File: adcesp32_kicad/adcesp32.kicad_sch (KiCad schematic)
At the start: 33 parts, among them IC1 PCM1862DBT, J1 AudioJack4, J2 USB_C_Receptacle_USB2.0_16P, J3 RCJ-2112, J4 Conn_01x05_Pin, J5 Conn_01x05_Pin, J6 Conn_01x04_Pin, J7 Conn_01x04_Pin, SW1 SW_Push, SW2 SW_Push, U1 ESP32-S3-WROOM-1, U2 AMS1117-3.3

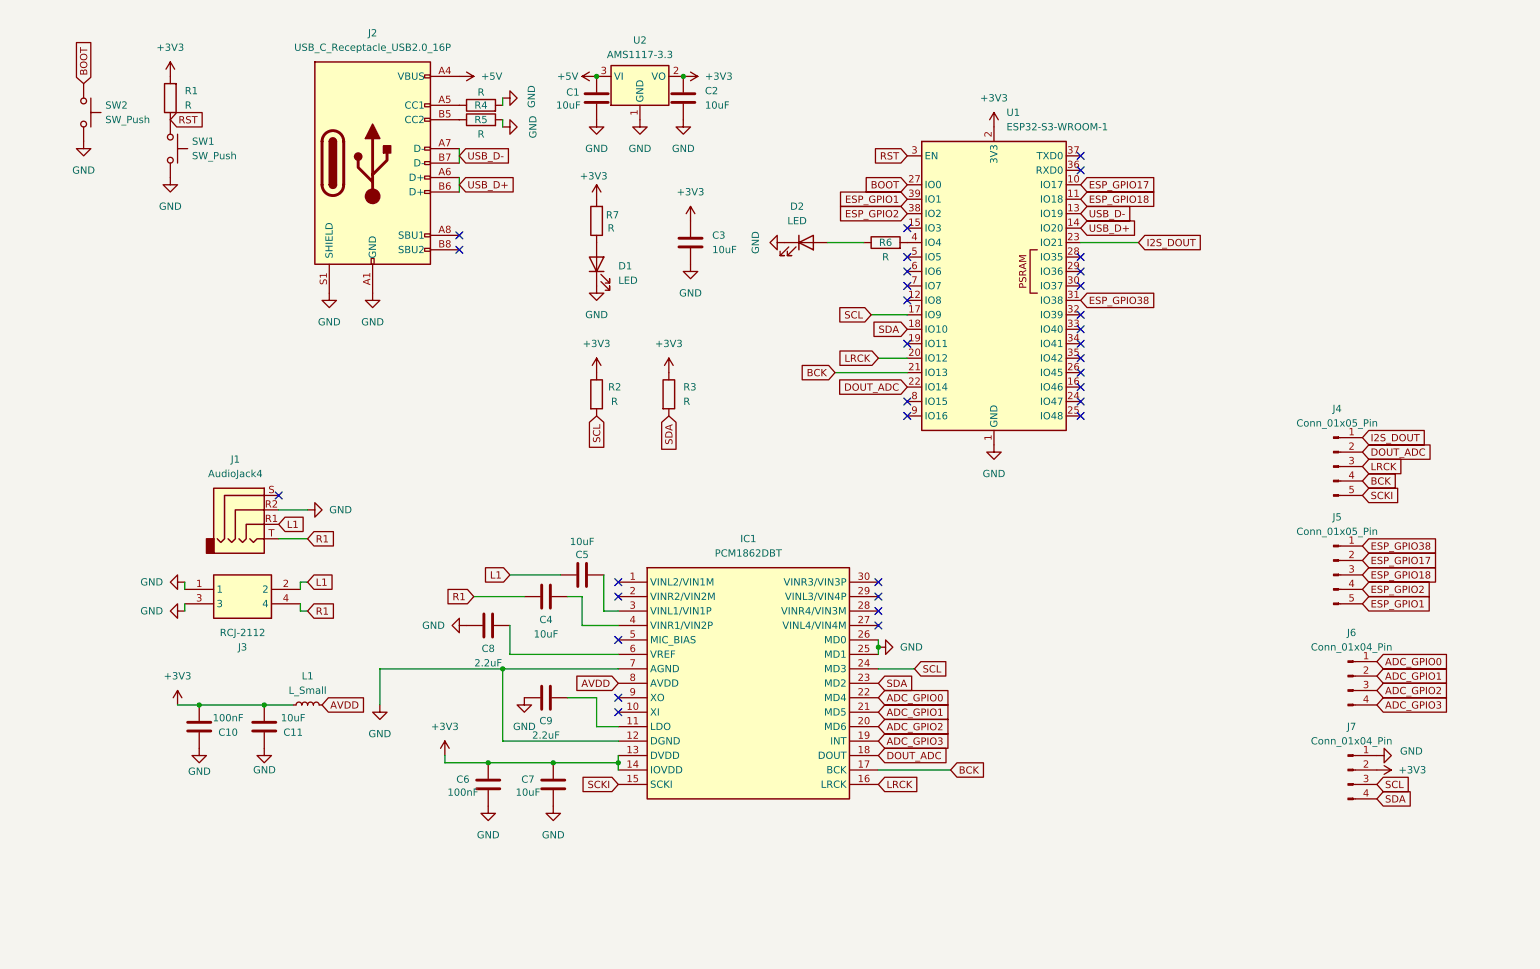
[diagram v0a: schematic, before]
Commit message: completed pcb design
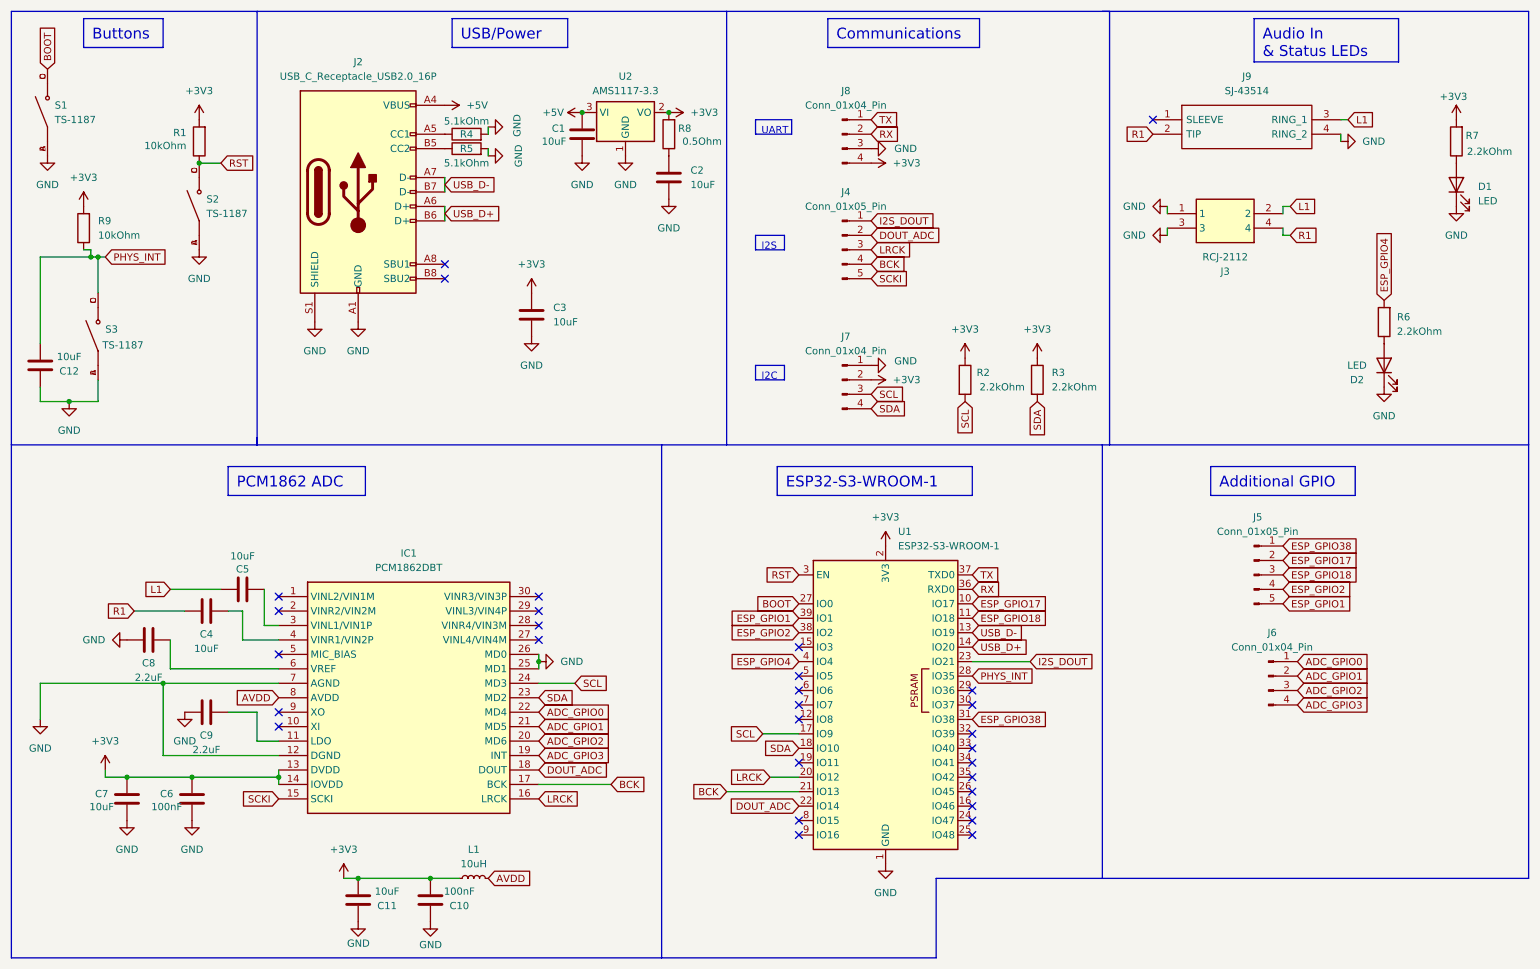
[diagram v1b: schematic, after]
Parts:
- removed J1: AudioJack4, symbol Connector_Audio:AudioJack4
- removed SW1, SW2: SW_Push, symbol Switch:SW_Push
- added C12: 10uF, Capacitor_SMD:C_0402_1005Metric, symbol Device:C
- added J8: Conn_01x04_Pin, Connector_PinHeader_1.00mm:PinHeader_1x04_P1.00mm_Vertical, symbol Connector:Conn_01x04_Pin
- added J9: SJ-43514, SJ43514, symbol SJ-43514:SJ-43514
- added R8: 0.5Ohm, Resistor_SMD:R_0603_1608Metric, symbol Device:R
- added R9: 10kOhm, Resistor_SMD:R_0402_1005Metric, symbol Device:R
- added S1, S2, S3: TS-1187, KiCad:SW_TS-1187A-B-A-B, symbol TS-1187A-B-A-B:TS-1187A-B-A-B
- D1, D2: footprint (none) -> Resistor_SMD:R_0805_2012Metric
- J2: footprint (none) -> Connector_USB:USB_C_Receptacle_HRO_TYPE-C-31-M-12
- L1: value L_Small -> 10uH; footprint (none) -> Inductor_SMD:L_0805_2012Metric
- R1: value R -> 10kOhm; footprint (none) -> Resistor_SMD:R_0402_1005Metric
- R2, R3, R6, R7: value R -> 2.2kOhm; footprint (none) -> Resistor_SMD:R_0603_1608Metric
- R4, R5: value R -> 5.1kOhm; footprint (none) -> Resistor_SMD:R_0402_1005Metric
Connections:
- net +3V3: now also J8.4 (Pin_4), R8.2, R9.2; no longer C2.1
- net BOOT: now also S1.C, S1.D
- net GND: now also C12.1, J8.3 (Pin_3), J9.4 (RING_2), S1.A, S1.B, S2.A, S2.B, S3.A, S3.B
- net L1: now also J9.3 (RING_1)
- net R1: now also J9.2 (TIP)
- net RST: now also S2.C, S2.D
- net PHYS_INT: now reaches U1.28 (IO35)
- net PHYS_INT: now also C12.2, R9.1, S3.C, S3.D
- net RX: now reaches U1.36 (RXD0)
- net RX: now also J8.2 (Pin_2)
- net TX: now reaches U1.37 (TXD0)
- net TX: now also J8.1 (Pin_1)
- net ESP_GPIO4: now reaches R6.2, U1.4 (IO4)
- new net: C2.1, R8.1
- no-connect marks 33 -> 30
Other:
- moved on the sheet: C1, C10, C11, C2, C3, C4, C5, C6, C7, C8, C9, D1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
